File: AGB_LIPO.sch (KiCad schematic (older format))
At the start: 4 parts, among them J1 Conn_01x02_Male, U1 tp4056_board-tp4056

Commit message: Load Sharing and Voltage stabilizer
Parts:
- removed U1: tp4056_board-tp4056, misc_footprints:4056E_LiIon_loader, symbol misc:tp4056_board-tp4056
- added Q1: Si2319CDS, Package_TO_SOT_SMD:SOT-23, symbol Transistor_FET:Si2319CDS
- added R1: 100K, Resistor_THT:R_Axial_DIN0309_L9.0mm_D3.2mm_P15.24mm_Horizontal, symbol Device:R
- added TP1: TestPoint, TestPoint:TestPoint_THTPad_D1.0mm_Drill0.5mm, symbol Connector:TestPoint
- added U1: misc_tp4056_board-tp4056, kiCad_mod:TP4056-18650, symbol AGB_LIPO:misc_tp4056_board-tp4056
- added U2: AMS1117-3.3, Package_TO_SOT_SMD:SOT-223-3_TabPin2, symbol Regulator_Linear:AMS1117-3.3
- D1: footprint misc_footprints:Diode-hybrid-3pad -> Diode_THT:D_DO-34_SOD68_P7.62mm_Horizontal
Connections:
- net labels added: 5v
- wire segments 17 -> 19
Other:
- moved on the sheet: J1
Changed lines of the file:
@@
 Comment4 ""
 $EndDescr
+Wire Wire Line
+	5250 3300 5200 3300
+Wire Wire Line
+	5200 3600 5250 3600
+Wire Wire Line
+	5250 3600 5250 3650
+NoConn ~ 4450 3500
+NoConn ~ 4450 3400
+Wire Wire Line
+	5250 2950 5250 3300
 $Comp
-L misc:tp4056_board-tp4056 U1
-U 1 1 5E2E0507
+L AGB_LIPO:misc_tp4056_board-tp4056 U1
+U 1 1 5EA05227
 P 4600 3200
 F 0 "U1" H 4825 3325 50  0000 C CNN
-F 1 "tp4056_board-tp4056" H 4825 3234 50  0000 C CNN
-F 2 "misc_footprints:4056E_LiIon_loader" H 4600 3200 50  0001 C CNN
+F 1 "misc_tp4056_board-tp4056" H 4825 3234 50  0000 C CNN
+F 2 "kiCad_mod:TP4056-18650" H 4600 3200 50  0001 C CNN
 F 3 "" H 4600 3200 50  0001 C CNN
 	1    4600 3200
@@
 $EndComp
 $Comp
-L Device:D D1
-U 1 1 5E2E0B2B
-P 5850 3250
-F 0 "D1" H 5850 3034 50  0000 C CNN
-F 1 "D" H 5850 3125 50  0000 C CNN
-F 2 "misc_footprints:Diode-hybrid-3pad" H 5850 3250 50  0001 C CNN
-F 3 "~" H 5850 3250 50  0001 C CNN
-	1    5850 3250
+L Device:R R1
+U 1 1 5EA0FDCF
+P 7000 2800
+F 0 "R1" H 7070 2846 50  0000 L CNN
+F 1 "100K" H 7070 2755 50  0000 L CNN
+F 2 "Resistor_THT:R_Axial_DIN0309_L9.0mm_D3.2mm_P15.24mm_Horizontal" V 6930 2800 50  0001 C CNN
+F 3 "~" H 7000 2800 50  0001 C CNN
+	1    7000 2800
+	1    0    0    -1
+$EndComp
+$Comp
+L Transistor_FET:Si2319CDS Q1
+U 1 1 5EA05791
+P 5900 2850
+F 0 "Q1" V 6149 2850 50  0000 C CNN
+F 1 "Si2319CDS" V 6240 2850 50  0000 C CNN
+F 2 "Package_TO_SOT_SMD:SOT-23" H 6100 2775 50  0001 L CIN
+F 3 "http://www.vishay.com/docs/66709/si2319cd.pdf" H 5900 2850 50  0001 L CNN
+	1    5900 2850
+	0    -1   1    0
+$EndComp
+Wire Wire Line
+	5350 3600 5600 3600
+Wire Wire Line
+	5350 3500 5350 3600
+Wire Wire Line
+	5200 3500 5350 3500
+Wire Wire Line
+	5350 3400 5200 3400
+Wire Wire Line
+	5350 3300 5350 3400
+Wire Wire Line
+	5600 3300 5350 3300
+$Comp
+L Connector:Conn_01x02_Male J1
+U 1 1 5E2E1CEE
+P 6900 3450
+F 0 "J1" H 6872 3332 50  0000 R CNN
+F 1 "Conn_01x02_Male" H 6872 3423 50  0000 R CNN
+F 2 "TestPoint:TestPoint_2Pads_Pitch2.54mm_Drill0.8mm" H 6900 3450 50  0001 C CNN
+F 3 "~" H 6900 3450 50  0001 C CNN
+	1    6900 3450
 	-1   0    0    1
 $EndComp
@@
 $EndComp
 $Comp
-L Connector:Conn_01x02_Male J1
-U 1 1 5E2E1CEE
-P 6450 3500
-F 0 "J1" H 6422 3382 50  0000 R CNN
-F 1 "Conn_01x02_Male" H 6422 3473 50  0000 R CNN
-F 2 "TestPoint:TestPoint_2Pads_Pitch2.54mm_Drill0.8mm" H 6450 3500 50  0001 C CNN
-F 3 "~" H 6450 3500 50  0001 C CNN
-	1    6450 3500
-	-1   0    0    1
+L Connector:TestPoint TP1
+U 1 1 5EA46751
+P 5900 2650
+F 0 "TP1" H 5958 2768 50  0000 L CNN
+F 1 "TestPoint" H 5958 2677 50  0000 L CNN
+F 2 "TestPoint:TestPoint_THTPad_D1.0mm_Drill0.5mm" H 6100 2650 50  0001 C CNN
+F 3 "~" H 6100 2650 50  0001 C CNN
+	1    5900 2650
+	1    0    0    -1
 $EndComp
 Wire Wire Line
-	5600 3300 5350 3300
+	7000 3650 7000 2950
+Connection ~ 5900 2650
+Connection ~ 6100 2650
 Wire Wire Line
-	5350 3300 5350 3400
+	6100 2650 5900 2650
+$Comp
+L Device:D D1
+U 1 1 5EA0E8EF
+P 6100 2800
+F 0 "D1" H 6100 2584 50  0000 C CNN
+F 1 "D" H 6100 2675 50  0000 C CNN
+F 2 "Diode_THT:D_DO-34_SOD68_P7.62mm_Horizontal" H 6100 2800 50  0001 C CNN
+F 3 "~" H 6100 2800 50  0001 C CNN
+	1    6100 2800
+	0    -1   -1   0
+$EndComp
+$Comp
+L Regulator_Linear:AMS1117-3.3 U2
+U 1 1 5EA50985
+P 6400 3350
+F 0 "U2" H 6400 3592 50  0000 C CNN
+F 1 "AMS1117-3.3" H 6400 3501 50  0000 C CNN
+F 2 "Package_TO_SOT_SMD:SOT-223-3_TabPin2" H 6400 3550 50  0001 C CNN
+F 3 "http://www.advanced-monolithic.com/pdf/ds1117.pdf" H 6500 3100 50  0001 C CNN
+	1    6400 3350
+	1    0    0    -1
+$EndComp
 Wire Wire Line
-	5350 3400 5200 3400
+	6400 3650 6700 3650
 Wire Wire Line
-	5200 3500 5350 3500
+	6700 3450 6700 3650
+Connection ~ 6700 3650
 Wire Wire Line
-	5350 3500 5350 3600
+	6700 3650 7000 3650
 Wire Wire Line
-	5350 3600 5600 3600
+	5250 3650 6400 3650
+Connection ~ 6400 3650
+Connection ~ 6100 2950
+Text Label 5900 2450 0    50   ~ 0
+5v
 Wire Wire Line
-	6250 3400 6150 3400
+	5250 2950 5700 2950
 Wire Wire Line
-	6150 3400 6150 3250
+	6100 2950 6100 3350
 Wire Wire Line
-	5250 3250 5250 3300
-Wire Wire Line
-	5250 3300 5200 3300
-Wire Wire Line
-	5200 3600 5250 3600
-Wire Wire Line
-	5250 3600 5250 3650
-Wire Wire Line
-	5250 3650 6150 3650
-Wire Wire Line
-	6150 3650 6150 3500
-Wire Wire Line
-	6150 3500 6250 3500
-Wire Wire Line
-	6000 3250 6150 3250
-Wire Wire Line
-	5700 3250 5250 3250
-NoConn ~ 4450 3500
-NoConn ~ 4450 3400
+	6100 2650 7000 2650
 $EndSCHEMATC

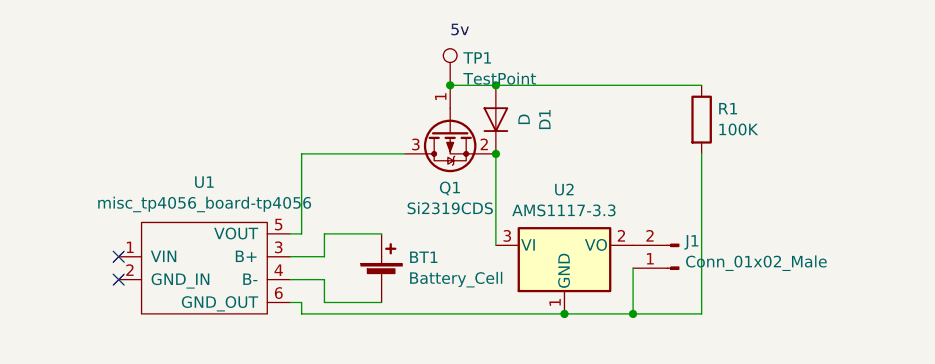
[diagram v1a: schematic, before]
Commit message: 29/04 Update
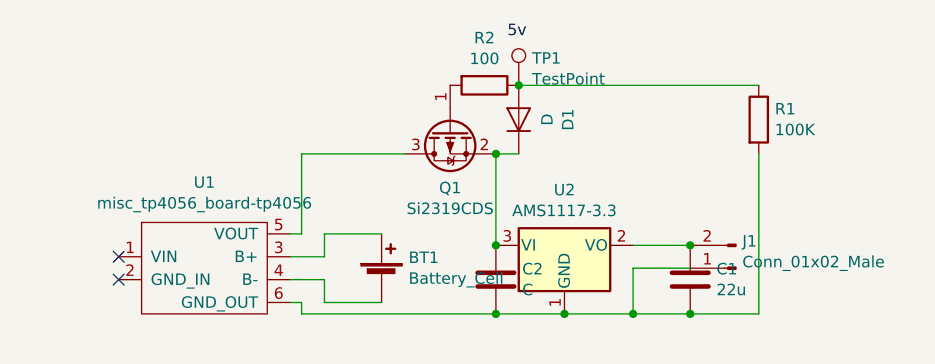
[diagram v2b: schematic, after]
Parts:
- added C1: 22u, Capacitor_Tantalum_SMD:CP_EIA-3216-18_Kemet-A, symbol Device:C
- added C2: C, Capacitor_Tantalum_SMD:CP_EIA-3216-18_Kemet-A, symbol Device:C
- added R2: 100, Resistor_THT:R_Axial_DIN0204_L3.6mm_D1.6mm_P7.62mm_Horizontal, symbol Device:R
- R1: footprint Resistor_THT:R_Axial_DIN0309_L9.0mm_D3.2mm_P15.24mm_Horizontal -> Resistor_THT:R_Axial_DIN0204_L3.6mm_D1.6mm_P7.62mm_Horizontal
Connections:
- net at J1.1 (Pin_1), R1.2, U1.6 (GND_OUT)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: now also C1.2, C2.2
- net at J1.2 (Pin_2), U2.2 (VO): now also C1.1
- net at D1.2 (A), R1.1, TP1.1: now also R2.1; no longer Q1.1 (G)
- net at D1.1 (K), Q1.2 (S), U2.3 (VI): now also C2.1
- new net: Q1.1 (G), R2.2
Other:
- moved on the sheet: D1, J1, R1, TP1
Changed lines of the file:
@@
 L Device:R R1
 U 1 1 5EA0FDCF
-P 7000 2800
-F 0 "R1" H 7070 2846 50  0000 L CNN
-F 1 "100K" H 7070 2755 50  0000 L CNN
-F 2 "Resistor_THT:R_Axial_DIN0309_L9.0mm_D3.2mm_P15.24mm_Horizontal" V 6930 2800 50  0001 C CNN
-F 3 "~" H 7000 2800 50  0001 C CNN
-	1    7000 2800
+P 7250 2800
+F 0 "R1" H 7320 2846 50  0000 L CNN
+F 1 "100K" H 7320 2755 50  0000 L CNN
+F 2 "Resistor_THT:R_Axial_DIN0204_L3.6mm_D1.6mm_P7.62mm_Horizontal" V 7180 2800 50  0001 C CNN
+F 3 "~" H 7250 2800 50  0001 C CNN
+	1    7250 2800
 	1    0    0    -1
 $EndComp
@@
 L Connector:Conn_01x02_Male J1
 U 1 1 5E2E1CEE
-P 6900 3450
-F 0 "J1" H 6872 3332 50  0000 R CNN
-F 1 "Conn_01x02_Male" H 6872 3423 50  0000 R CNN
-F 2 "TestPoint:TestPoint_2Pads_Pitch2.54mm_Drill0.8mm" H 6900 3450 50  0001 C CNN
-F 3 "~" H 6900 3450 50  0001 C CNN
-	1    6900 3450
+P 7150 3450
+F 0 "J1" H 7122 3332 50  0000 R CNN
+F 1 "Conn_01x02_Male" H 7122 3423 50  0000 R CNN
+F 2 "TestPoint:TestPoint_2Pads_Pitch2.54mm_Drill0.8mm" H 7150 3450 50  0001 C CNN
+F 3 "~" H 7150 3450 50  0001 C CNN
+	1    7150 3450
 	-1   0    0    1
 $EndComp
@@
 L Connector:TestPoint TP1
 U 1 1 5EA46751
-P 5900 2650
-F 0 "TP1" H 5958 2768 50  0000 L CNN
-F 1 "TestPoint" H 5958 2677 50  0000 L CNN
-F 2 "TestPoint:TestPoint_THTPad_D1.0mm_Drill0.5mm" H 6100 2650 50  0001 C CNN
-F 3 "~" H 6100 2650 50  0001 C CNN
-	1    5900 2650
+P 6200 2650
+F 0 "TP1" H 6258 2768 50  0000 L CNN
+F 1 "TestPoint" H 6258 2677 50  0000 L CNN
+F 2 "TestPoint:TestPoint_THTPad_D1.0mm_Drill0.5mm" H 6400 2650 50  0001 C CNN
+F 3 "~" H 6400 2650 50  0001 C CNN
+	1    6200 2650
 	1    0    0    -1
 $EndComp
 Wire Wire Line
-	7000 3650 7000 2950
-Connection ~ 5900 2650
-Connection ~ 6100 2650
-Wire Wire Line
-	6100 2650 5900 2650
+	7250 3650 7250 2950
 $Comp
 L Device:D D1
 U 1 1 5EA0E8EF
-P 6100 2800
-F 0 "D1" H 6100 2584 50  0000 C CNN
-F 1 "D" H 6100 2675 50  0000 C CNN
-F 2 "Diode_THT:D_DO-34_SOD68_P7.62mm_Horizontal" H 6100 2800 50  0001 C CNN
-F 3 "~" H 6100 2800 50  0001 C CNN
-	1    6100 2800
+P 6200 2800
+F 0 "D1" H 6200 2584 50  0000 C CNN
+F 1 "D" H 6200 2675 50  0000 C CNN
+F 2 "Diode_THT:D_DO-34_SOD68_P7.62mm_Horizontal" H 6200 2800 50  0001 C CNN
+F 3 "~" H 6200 2800 50  0001 C CNN
+	1    6200 2800
 	0    -1   -1   0
 $EndComp
@@
 Wire Wire Line
 	6700 3450 6700 3650
-Connection ~ 6700 3650
 Wire Wire Line
-	6700 3650 7000 3650
-Wire Wire Line
-	5250 3650 6400 3650
+	5250 3650 6100 3650
 Connection ~ 6400 3650
-Connection ~ 6100 2950
-Text Label 5900 2450 0    50   ~ 0
+Text Label 6150 2450 0    50   ~ 0
 5v
 Wire Wire Line
@@
 Wire Wire Line
 	6100 2950 6100 3350
+$Comp
+L Device:R R2
+U 1 1 5EA6A02A
+P 6050 2650
+F 0 "R2" V 5843 2650 50  0000 C CNN
+F 1 "100" V 5934 2650 50  0000 C CNN
+F 2 "Resistor_THT:R_Axial_DIN0204_L3.6mm_D1.6mm_P7.62mm_Horizontal" V 5980 2650 50  0001 C CNN
+F 3 "~" H 6050 2650 50  0001 C CNN
+	1    6050 2650
+	0    1    1    0
+$EndComp
+Connection ~ 6200 2650
 Wire Wire Line
-	6100 2650 7000 2650
+	6100 2950 6200 2950
+Connection ~ 6100 2950
+Wire Wire Line
+	6700 3650 6950 3650
+Connection ~ 6700 3650
+Wire Wire Line
+	6700 3450 6950 3450
+Wire Wire Line
+	6200 2650 7250 2650
+$Comp
+L Device:C C1
+U 1 1 5EA99052
+P 6950 3500
+F 0 "C1" H 7065 3546 50  0000 L CNN
+F 1 "22u" H 7065 3455 50  0000 L CNN
+F 2 "Capacitor_Tantalum_SMD:CP_EIA-3216-18_Kemet-A" H 6988 3350 50  0001 C CNN
+F 3 "~" H 6950 3500 50  0001 C CNN
+	1    6950 3500
+	1    0    0    -1
+$EndComp
+Connection ~ 6950 3650
+Wire Wire Line
+	6950 3650 7250 3650
+Wire Wire Line
+	6950 3350 6700 3350
+Connection ~ 6950 3350
+$Comp
+L Device:C C2
+U 1 1 5EA9D6A6
+P 6100 3500
+F 0 "C2" H 6215 3546 50  0000 L CNN
+F 1 "C" H 6215 3455 50  0000 L CNN
+F 2 "Capacitor_Tantalum_SMD:CP_EIA-3216-18_Kemet-A" H 6138 3350 50  0001 C CNN
+F 3 "~" H 6100 3500 50  0001 C CNN
+	1    6100 3500
+	1    0    0    -1
+$EndComp
+Connection ~ 6100 3350
+Connection ~ 6100 3650
+Wire Wire Line
+	6100 3650 6400 3650
 $EndSCHEMATC
